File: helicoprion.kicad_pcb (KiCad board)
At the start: 2 copper layers, 151.8 x 125.7 mm, 58 parts, among them J1 TRRS, J2 TRRS, SW1 SW_SPST, SW10 SW_SPST, SW11 SW_SPST, SW12 SW_SPST, SW13 SW_SPST, SW14 SW_SPST, SW15 SW_SPST, SW16 SW_SPST, SW17 SW_SPST, SW18 SW_SPST, SW19 SW_SPST, SW2 SW_SPST, SW20 SW_SPST, SW21 SW_SPST, SW22 SW_SPST, SW23 SW_SPST, SW24 SW_SPST, SW25 SW_SPST, SW26 SW_SPST, SW3 SW_SPST, SW4 SW_SPST, SW5 SW_SPST, SW6 SW_SPST, SW7 SW_SPST, SW8 SW_SPST, SW9 SW_SPST, U1 ProMicro_r

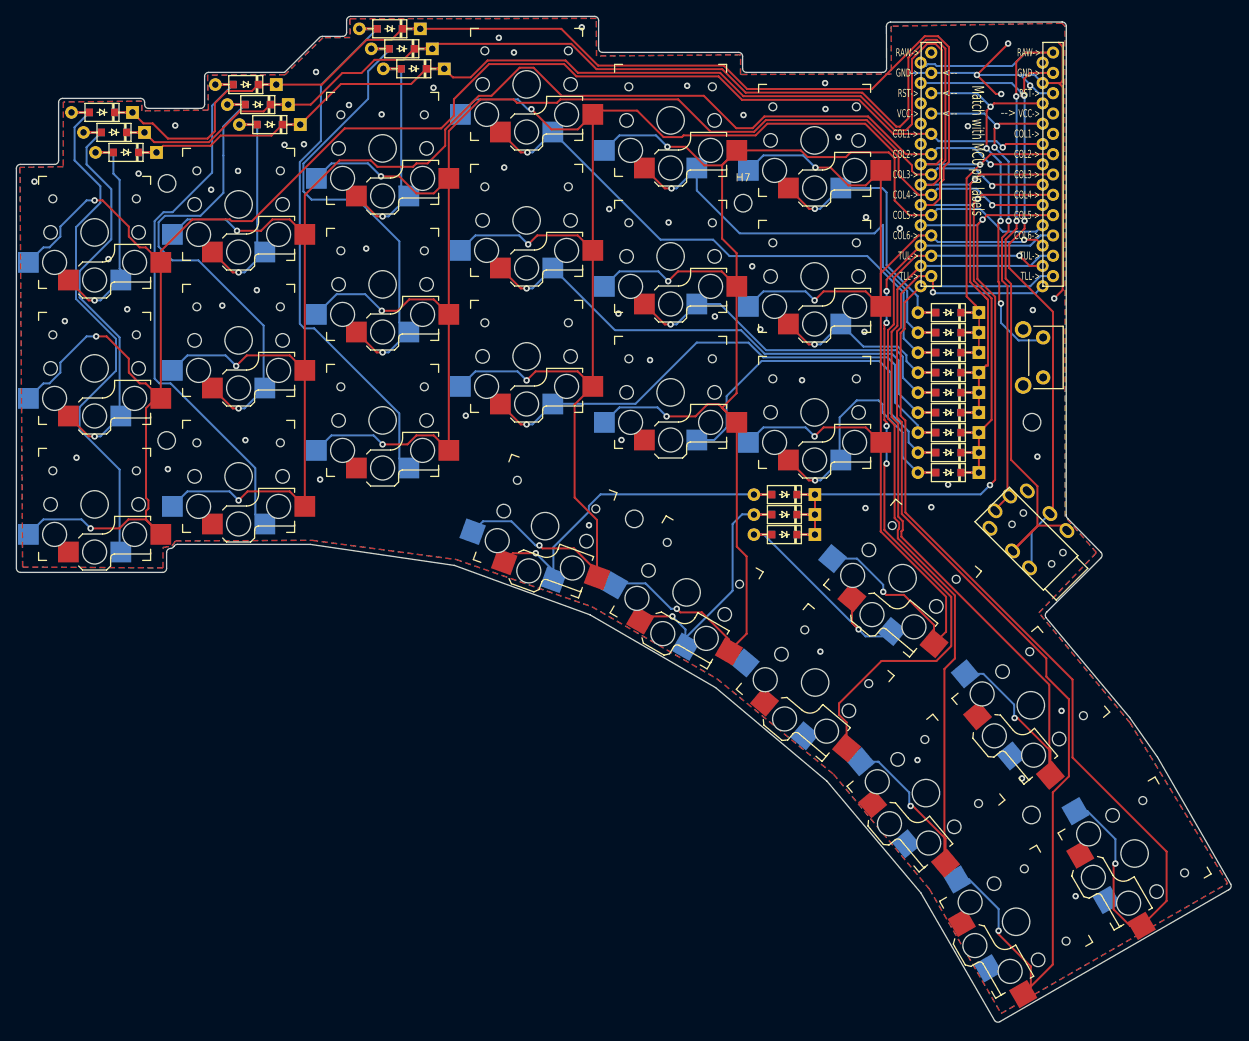
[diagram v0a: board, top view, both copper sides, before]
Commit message: finish layout
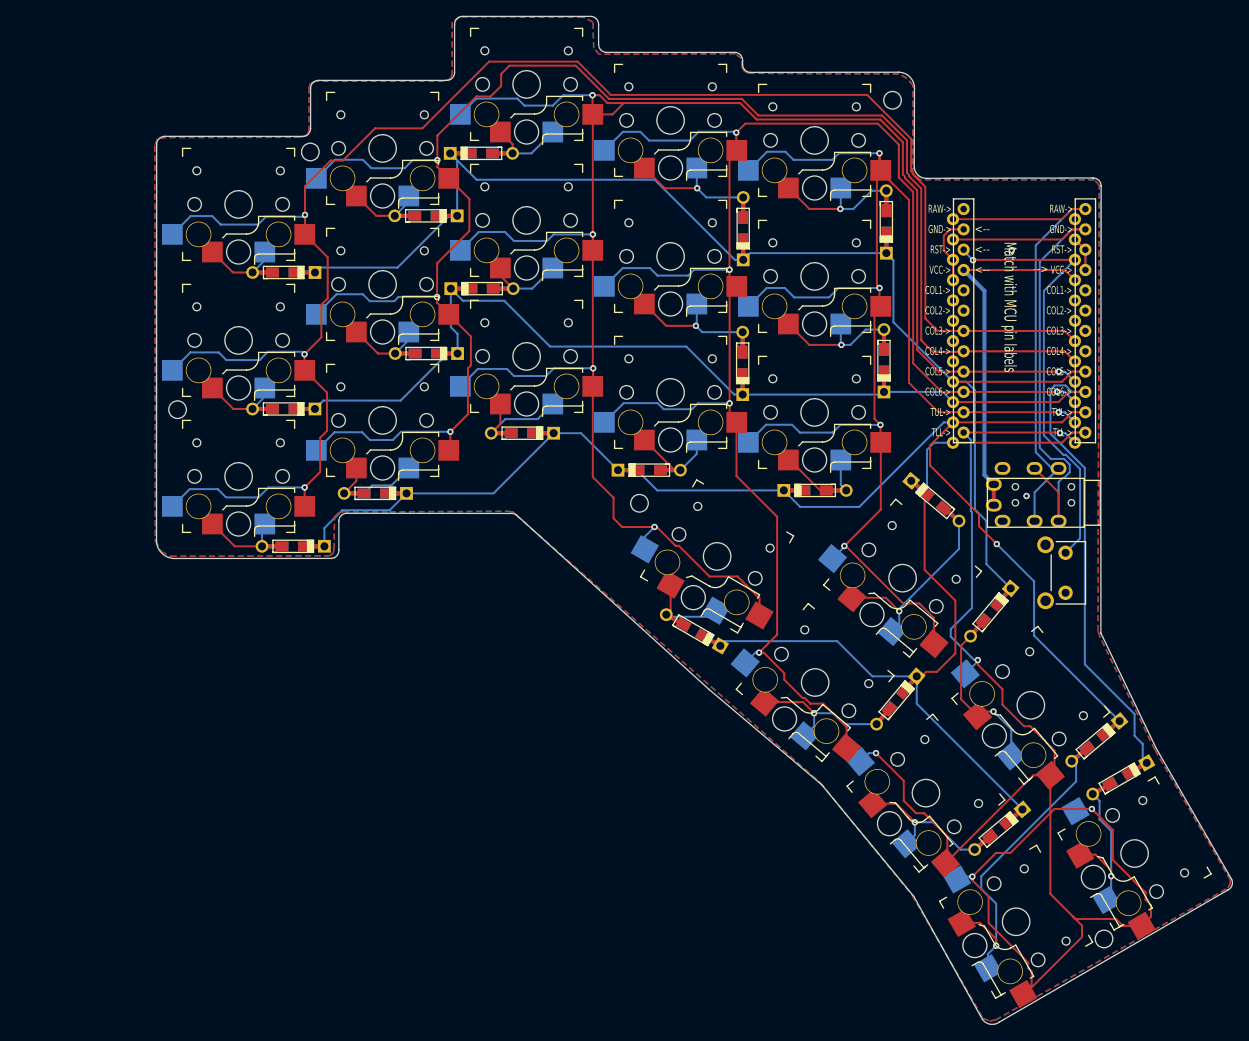
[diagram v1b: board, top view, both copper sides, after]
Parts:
- removed D24, D25, D26: 1N4148, various:double_sided_hybrid_sod123_tht
- removed H6, H7: MountingHole, MountingHole:MountingHole_2.2mm_M2
- removed SW24, SW25, SW26, SW8: SW_SPST, keyswitches:Kailh_socket_PG1350_reversible
- added D3: 1N4148, Keebio-Parts:Diode-dual, F.Cu at (165.5, 97.0)
- added D4: 1N4148, Keebio-Parts:Diode-dual, F.Cu at (181.6, 117.8)
- added D5: 1N4148, Keebio-Parts:Diode-dual, F.Cu at (178.6, 113.1)
- added D7: 1N4148, Keebio-Parts:Diode-dual, F.Cu at (166.5, 124.1)
- D1, D10, D11, D12, D13, D14, D15, D16, D17, D18, D19, D2, D20, D21, D22, D23, D6, D9: footprint various:double_sided_hybrid_sod123_tht -> Keebio-Parts:Diode-dual
- moved D15 63.5 mm to (101.8, 39.6)
- moved D16 60.3 mm to (101.9, 56.5)
- moved D20 58.1 mm to (88.6, 82.1), turned to 0 degrees
- moved D23 58.0 mm to (78.3, 88.7), turned to 0 degrees
- moved D17 53.2 mm to (107.0, 74.6), turned to 0 degrees
- moved H4 50.1 mm to (121.6, 83.4)
- moved D19 38.2 mm to (95.0, 64.6), turned to 0 degrees
- moved D22 38.2 mm to (77.1, 71.6), turned to 0 degrees
- moved D14 37.5 mm to (122.8, 79.2)
- moved D12 28.7 mm to (134.6, 49.0), turned to -90 degrees
- moved D2 27.1 mm to (153.8, 108.0), turned to 50 degrees
- moved RSW1 27.1 mm to (173.6, 92.0)
- moved D13 26.0 mm to (134.5, 65.9), turned to -90 degrees
- moved D1 20.4 mm to (128.3, 99.2), turned to -30 degrees
- moved U1 20.0 mm to (169.7, 61.1)
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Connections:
- SW1 pad 1: Net-(D2-A) -> Net-(D1-A)
- SW1 pad 2: col2 -> col4
- SW10 pad 2: col1 -> col2
- SW11 pad 2: col1 -> col2
- SW12 pad 2: col2 -> col3
- SW13 pad 2: col2 -> col3
- SW14 pad 2: col2 -> col3
- SW15 pad 2: col3 -> col4
- SW16 pad 2: col3 -> col4
- SW17 pad 2: col3 -> col4
- SW18 pad 2: col4 -> col5
- SW19 pad 2: col4 -> col5
- SW2 pad 1: GND -> Net-(D2-A)
- SW2 pad 2: tum -> col3
- SW20 pad 2: col4 -> col5
- SW21 pad 2: col5 -> col6
- SW22 pad 2: col5 -> col6
- SW23 pad 2: col5 -> col6
- SW3 pad 2: col1 -> col2
- SW4 pad 1: GND -> Net-(D7-A)
- SW4 pad 2: tll -> col1
- SW5 pad 1: GND -> Net-(D3-A)
- SW5 pad 2: tul -> col1
- SW6 pad 1: GND -> Net-(D5-A)
- SW6 pad 2: tlr -> col1
- SW7 pad 1: GND -> Net-(D4-A)
- SW7 pad 2: tur -> col1
- SW9 pad 2: col1 -> col2
- U1 pad 10: tum -> row2
- U1 pad 11: tul -> row3
- U1 pad 12: tur -> row4
- U1 pad 13: tlr -> col1
- U1 pad 14: tll -> col2
- U1 pad 15: col1 -> col3
- U1 pad 16: col2 -> col4
- U1 pad 17: col3 -> col5
- U1 pad 18: col4 -> col6
- U1 pad 19: col5 -> unconnected-(U1-A2/F5-Pad19)
- U1 pad 20: col6 -> unconnected-(U1-A3/F4-Pad20)
- U1 pad 6: row1 -> unconnected-(U1-SCL/D0/3-Pad6)
- U1 pad 7: row2 -> unconnected-(U1-D4/4-Pad7)
- U1 pad 8: row3 -> unconnected-(U1-C6/5-Pad8)
- U1 pad 9: row4 -> row1
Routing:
- net tlr: track 139.4 -> 0.00 mm, vias 2 -> 0
- net tur: track 132.8 -> 0.00 mm, vias 1 -> 0
- net tll: track 116.5 -> 0.00 mm, vias 2 -> 0
- net tul: track 109.2 -> 0.00 mm, vias 1 -> 0
- net tum: track 95.7 -> 0.00 mm, vias 4 -> 0
- net Net-(D26-A): track 64.4 -> 0.00 mm
- net Net-(D15-A): track 69.0 -> 9.43 mm, vias 1 -> 0
- net Net-(D23-A): track 66.2 -> 10.3 mm
- net Net-(D16-A): track 64.0 -> 9.26 mm, vias 1 -> 0
- net Net-(D20-A): track 65.3 -> 10.7 mm
- net Net-(D17-A): track 65.4 -> 13.3 mm, vias 1 -> 0
- net Net-(D25-A): track 49.9 -> 0.00 mm, vias 1 -> 0
- net GND: track 66.9 -> 17.6 mm, vias 60 -> 2
- net Net-(D22-A): track 58.6 -> 9.36 mm, vias 1 -> 0
- net col4: track 181.4 -> 230.4 mm, vias 4 -> 5
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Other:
- board size 151.8 x 125.7 mm -> 134.5 x 126 mm
